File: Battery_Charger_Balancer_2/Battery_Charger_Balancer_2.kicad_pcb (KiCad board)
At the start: 2 copper layers, 36 x 65 mm, 120 parts, among them J1 GSB1C41110SSHR, J2 Conn_02x03_Odd_Even, J3 Conn_01x06_Pin, J4 Conn_01x02_Socket, J5 Conn_01x02_Socket, J6 Conn_01x02_Pin, Q1 GSFD0646, SW1 SW_SPDT, U1 RT1719GQW, U10 BAV74_215, U2 SSF3611E, U3 ETA3000D2I, U4 BQ25690RBAR, U5 ETA3000D2I, U6 ETA3000D2I, U8 ETA3000D2I, U9 TCR1HF33B

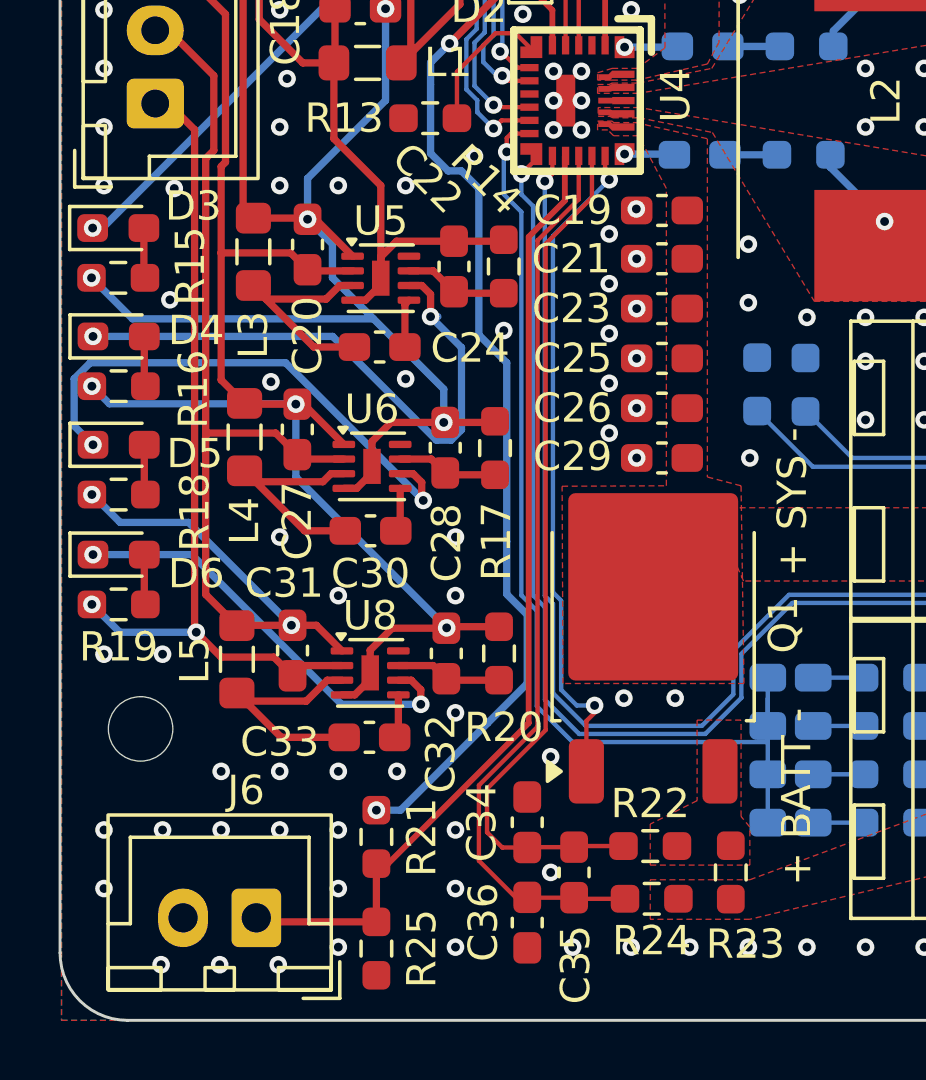
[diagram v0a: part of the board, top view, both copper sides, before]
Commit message: Updates after production of first rev
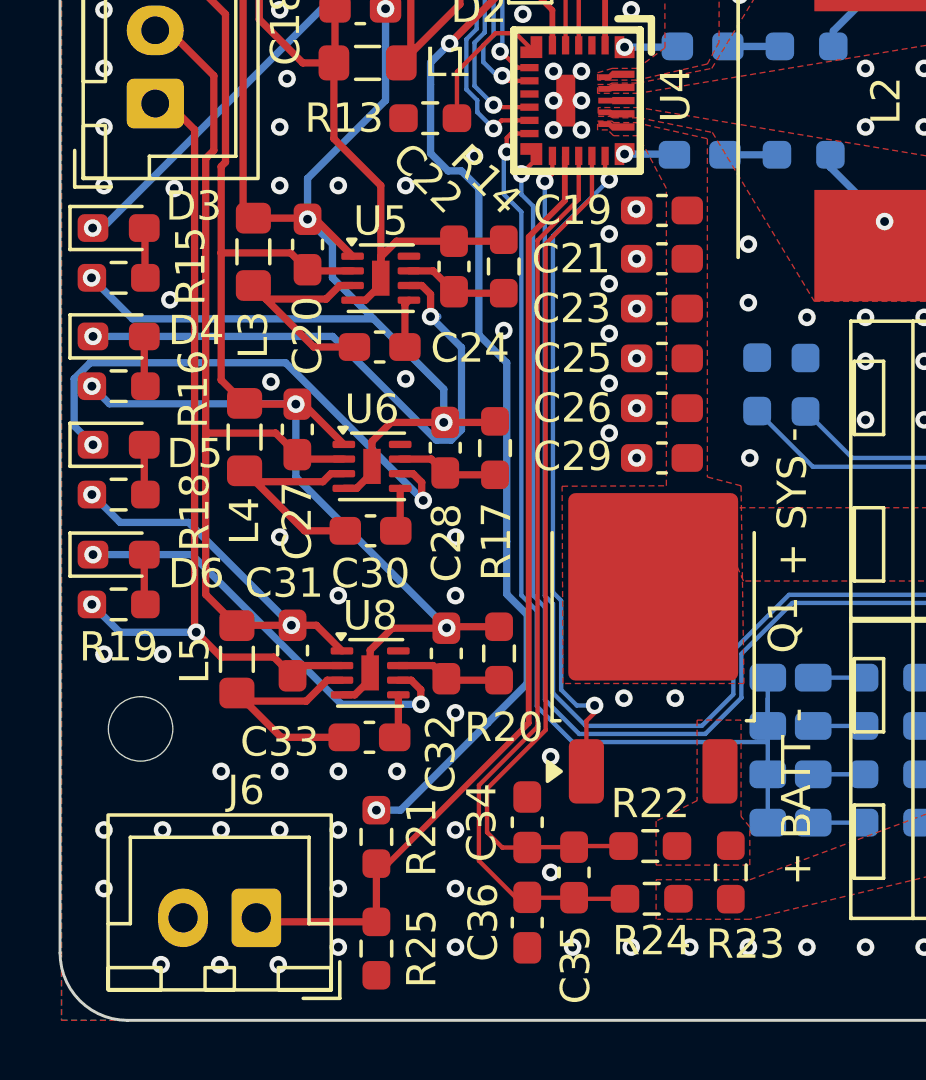
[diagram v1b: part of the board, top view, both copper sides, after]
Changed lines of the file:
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@@
 	(footprint "LED_SMD:LED_0603_1608Metric_Pad1.05x0.95mm_HandSolder"
 		(layer "F.Cu")
-		(at 13.9875 49.95)
+		(at 14 49.95)
 		(descr "LED SMD 0603 (1608 Metric), square (rectangular) end terminal, IPC-7351 nominal, (Body size source: http://www.tortai-tech.com/upload/download/2011102023233369053.pdf), generated with kicad-footprint-generator")
 		(tags "LED handsolder")
@@
 	(footprint "Resistor_SMD:R_0603_1608Metric_Pad0.98x0.95mm_HandSolder"
 		(layer "F.Cu")
-		(at 13.9875 51.65)
+		(at 14 51.65)
 		(descr "Resistor SMD 0603 (1608 Metric), square (rectangular) end terminal, IPC-7351 nominal with elongated pad for handsoldering. (Body size source: IPC-SM-782 page 72, https://www.pcb-3d.com/wordpress/wp-content/uploads/ipc-sm-782a_amendment_1_and_2.pdf), generated with kicad-footprint-generator")
 		(tags "resistor handsolder")
@@
 	(segment
 		(start 14.8625 49.95)
-		(end 14.8625 51.6125)
+		(end 14.9 49.9875)
 		(width 0.25)
 		(layer "F.Cu")
@@
 	)
 	(segment
-		(start 14.8625 51.6125)
+		(start 14.9 49.9875)
 		(end 14.9 51.65)
 		(width 0.25)
@@
 		(polygon
 			(pts
-				(xy 35.25 66.75) (xy 33.75 66.75) (xy 33.75 69.5) (xy 32.15 70.3) (xy 32.15 71.7) (xy 35.55 71.7)
+				(xy 35.25 66.75) (xy 33.75 66.75) (xy 33.75 69.5) (xy 32.35 70.2) (xy 32.35 71.7) (xy 35.55 71.7)
 				(xy 35.55 70.4) (xy 35.25 70.037931)
 			)
@@
 		(polygon
 			(pts
-				(xy 32.15 72.2) (xy 35.55 72.2) (xy 42 69.8) (xy 44.4 69.8) (xy 44.4 72) (xy 42 72) (xy 35.55 73.55)
-				(xy 32.15 73.55)
+				(xy 32.35 72.2) (xy 35.55 72.2) (xy 42 69.8) (xy 44.4 69.8) (xy 44.4 72) (xy 42 72) (xy 35.55 73.55)
+				(xy 32.35 73.55)
 			)
 		)
